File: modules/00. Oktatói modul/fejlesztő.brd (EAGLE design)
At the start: 77.5 x 22.5 mm, 22 parts

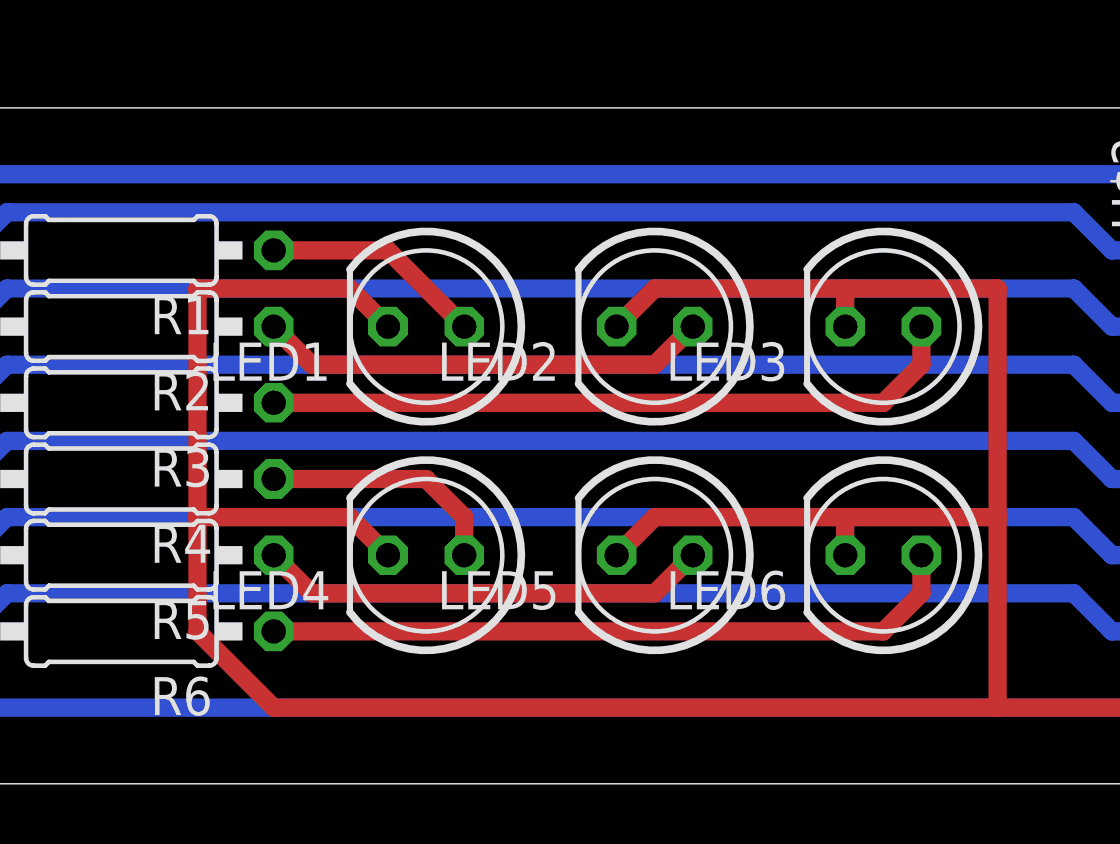
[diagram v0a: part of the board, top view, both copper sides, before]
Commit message: Added most CAM files
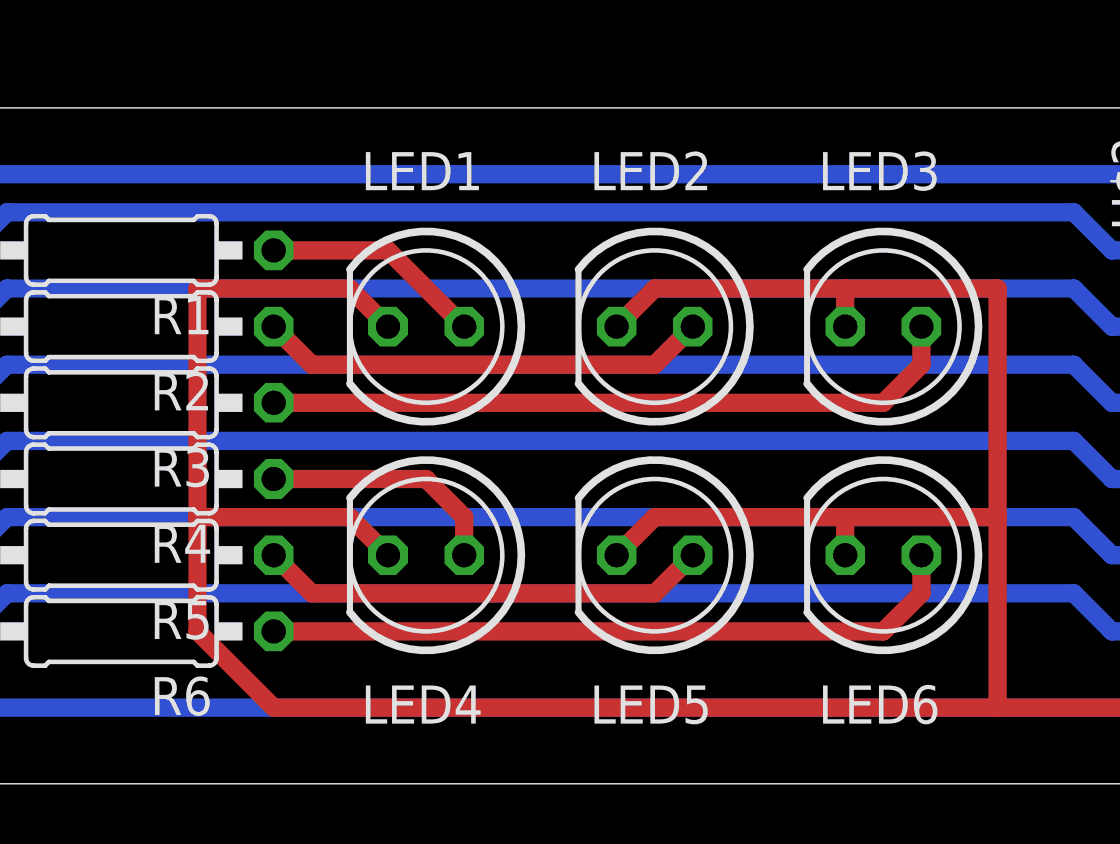
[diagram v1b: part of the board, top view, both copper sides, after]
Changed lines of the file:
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@@
 <?xml version="1.0" encoding="utf-8"?>
 <!DOCTYPE eagle SYSTEM "eagle.dtd">
-<eagle version="6.5.0">
+<eagle version="9.0.0">
 <drawing>
 <settings>
 <setting alwaysvectorfont="no"/>
+<setting keepoldvectorfont="yes"/>
 <setting verticaltext="up"/>
 </settings>
@@
 <param name="dpMaxLengthDifference" value="10mm"/>
 <param name="dpGapFactor" value="2.5"/>
-<param name="checkGrid" value="0"/>
 <param name="checkAngle" value="0"/>
 <param name="checkFont" value="1"/>
 <param name="checkRestrict" value="1"/>
+<param name="checkStop" value="0"/>
+<param name="checkValues" value="0"/>
 <param name="useDiameter" value="13"/>
 <param name="maxErrors" value="50"/>
@@
 <pass name="Default">
 <param name="RoutingGrid" value="50mil"/>
+<param name="AutoGrid" value="1"/>
+<param name="Efforts" value="0"/>
+<param name="TopRouterVariant" value="1"/>
 <param name="tpViaShape" value="round"/>
 <param name="PrefDir.1" value="|"/>
@@
 <element name="IO1" library="wirepad" package="2,15/1,0" value="" x="22.86" y="17.78"/>
 <element name="R1" library="resistor" package="0207/10" value="180" x="38.1" y="17.78" rot="R180"/>
-<element name="LED1" library="led" package="LED5MM" value="" x="48.26" y="15.24" rot="R180"/>
+<element name="LED1" library="led" package="LED5MM" value="" x="48.26" y="15.24" smashed="yes" rot="R180">
+<attribute name="NAME" x="50.165" y="21.0566" size="1.27" layer="25" ratio="10" rot="R180"/>
+<attribute name="VALUE" x="45.0596" y="17.0434" size="1.27" layer="27" ratio="10" rot="R180"/>
+</element>
 <element name="IO2" library="wirepad" package="2,15/1,0" value="" x="22.86" y="15.24"/>
 <element name="R2" library="resistor" package="0207/10" value="180" x="38.1" y="15.24" rot="R180"/>
-<element name="LED2" library="led" package="LED5MM" value="" x="55.88" y="15.24" rot="R180"/>
+<element name="LED2" library="led" package="LED5MM" value="" x="55.88" y="15.24" smashed="yes" rot="R180">
+<attribute name="NAME" x="57.785" y="21.0566" size="1.27" layer="25" ratio="10" rot="R180"/>
+<attribute name="VALUE" x="52.6796" y="17.0434" size="1.27" layer="27" ratio="10" rot="R180"/>
+</element>
 <element name="IO3" library="wirepad" package="2,15/1,0" value="" x="22.86" y="12.7"/>
 <element name="R3" library="resistor" package="0207/10" value="180" x="38.1" y="12.7" rot="R180"/>
-<element name="LED3" library="led" package="LED5MM" value="" x="63.5" y="15.24" rot="R180"/>
+<element name="LED3" library="led" package="LED5MM" value="" x="63.5" y="15.24" smashed="yes" rot="R180">
+<attribute name="NAME" x="65.405" y="21.0566" size="1.27" layer="25" ratio="10" rot="R180"/>
+<attribute name="VALUE" x="60.2996" y="17.0434" size="1.27" layer="27" ratio="10" rot="R180"/>
+</element>
 <element name="IO4" library="wirepad" package="2,15/1,0" value="" x="22.86" y="10.16"/>
 <element name="R4" library="resistor" package="0207/10" value="180" x="38.1" y="10.16" rot="R180"/>
-<element name="LED4" library="led" package="LED5MM" value="" x="48.26" y="7.62" rot="R180"/>
+<element name="LED4" library="led" package="LED5MM" value="" x="48.26" y="7.62" smashed="yes" rot="R180">
+<attribute name="NAME" x="50.165" y="3.2766" size="1.27" layer="25" ratio="10" rot="R180"/>
+<attribute name="VALUE" x="45.0596" y="9.4234" size="1.27" layer="27" ratio="10" rot="R180"/>
+</element>
 <element name="IO5" library="wirepad" package="2,15/1,0" value="" x="22.86" y="7.62"/>
 <element name="R5" library="resistor" package="0207/10" value="180" x="38.1" y="7.62" rot="R180"/>
-<element name="LED5" library="led" package="LED5MM" value="" x="55.88" y="7.62" rot="R180"/>
+<element name="LED5" library="led" package="LED5MM" value="" x="55.88" y="7.62" smashed="yes" rot="R180">
+<attribute name="NAME" x="57.785" y="3.2766" size="1.27" layer="25" ratio="10" rot="R180"/>
+<attribute name="VALUE" x="52.6796" y="9.4234" size="1.27" layer="27" ratio="10" rot="R180"/>
+</element>
 <element name="IO6" library="wirepad" package="2,15/1,0" value="" x="22.86" y="5.08"/>
 <element name="R6" library="resistor" package="0207/10" value="180" x="38.1" y="5.08" rot="R180"/>
-<element name="LED6" library="led" package="LED5MM" value="" x="63.5" y="7.62" rot="R180"/>
+<element name="LED6" library="led" package="LED5MM" value="" x="63.5" y="7.62" smashed="yes" rot="R180">
+<attribute name="NAME" x="65.405" y="3.2766" size="1.27" layer="25" ratio="10" rot="R180"/>
+<attribute name="VALUE" x="60.2996" y="9.4234" size="1.27" layer="27" ratio="10" rot="R180"/>
+</element>
 </elements>
 <signals>
